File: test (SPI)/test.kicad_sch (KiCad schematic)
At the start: 22 parts, among them J1 Conn_01x02, J2 Conn_01x02, J3 Conn_01x10, U1 DRV8873SPWPRQ1

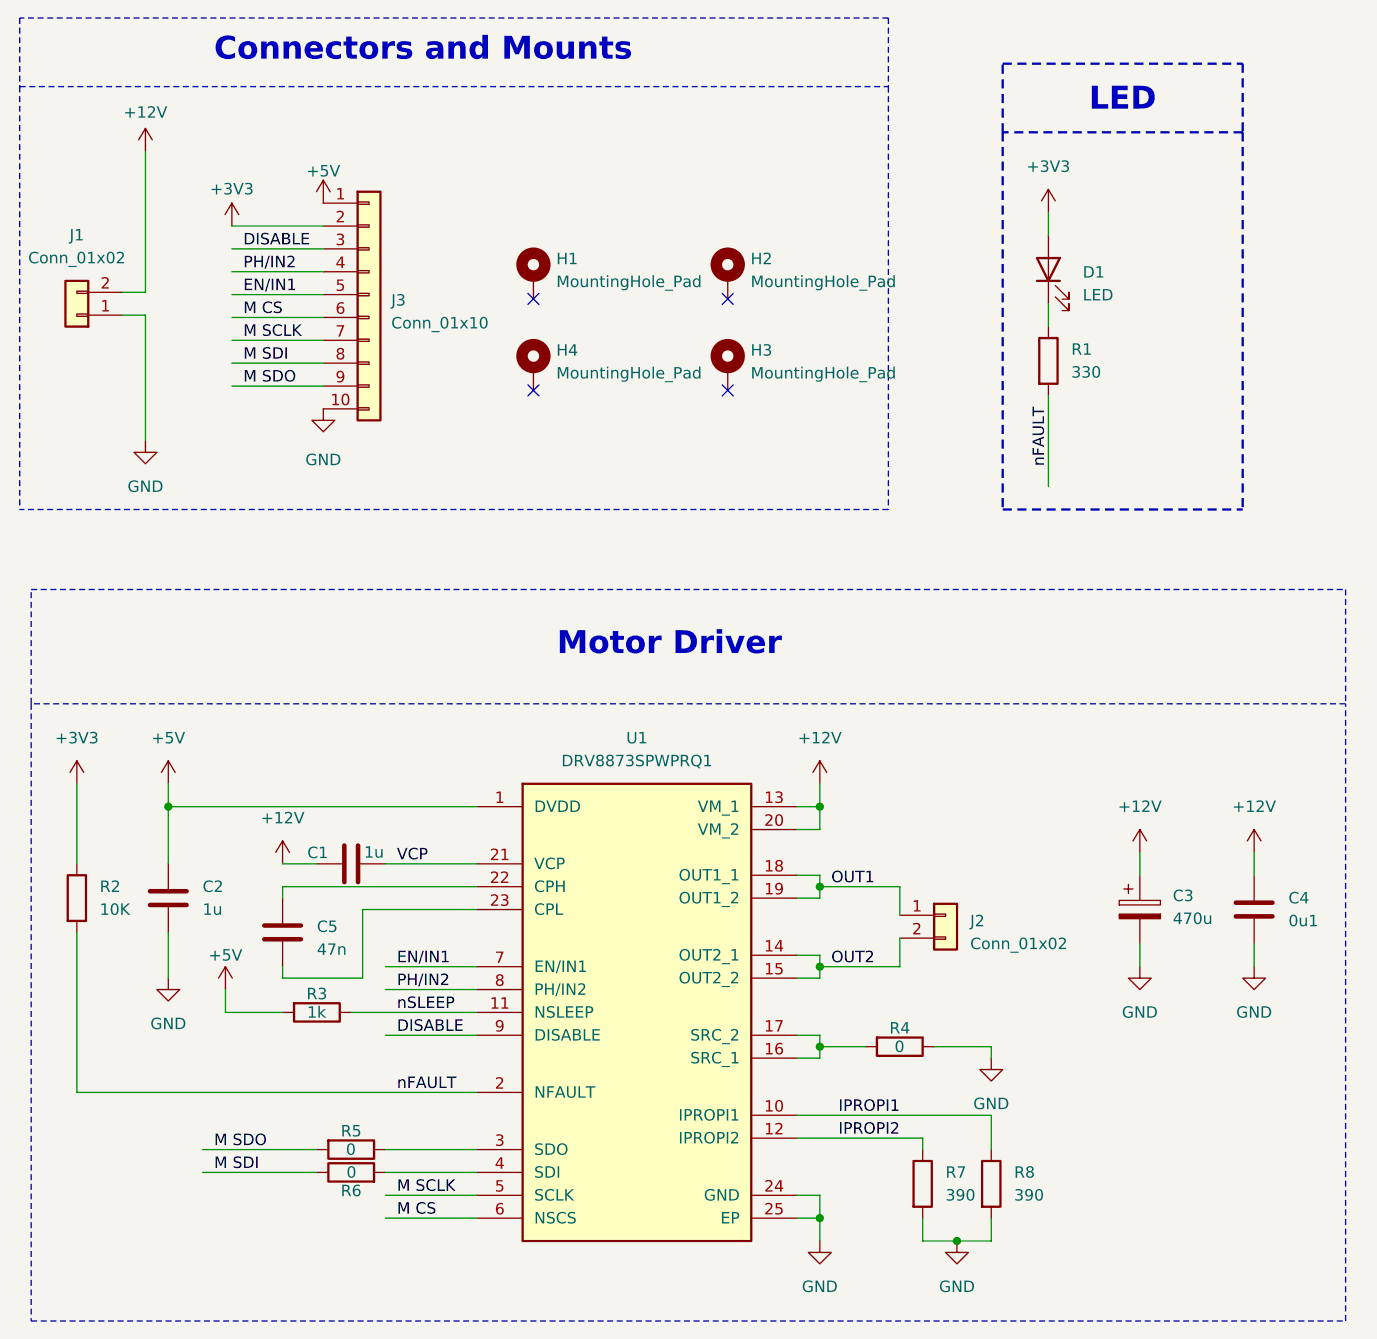
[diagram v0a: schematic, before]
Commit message: Test PCBS
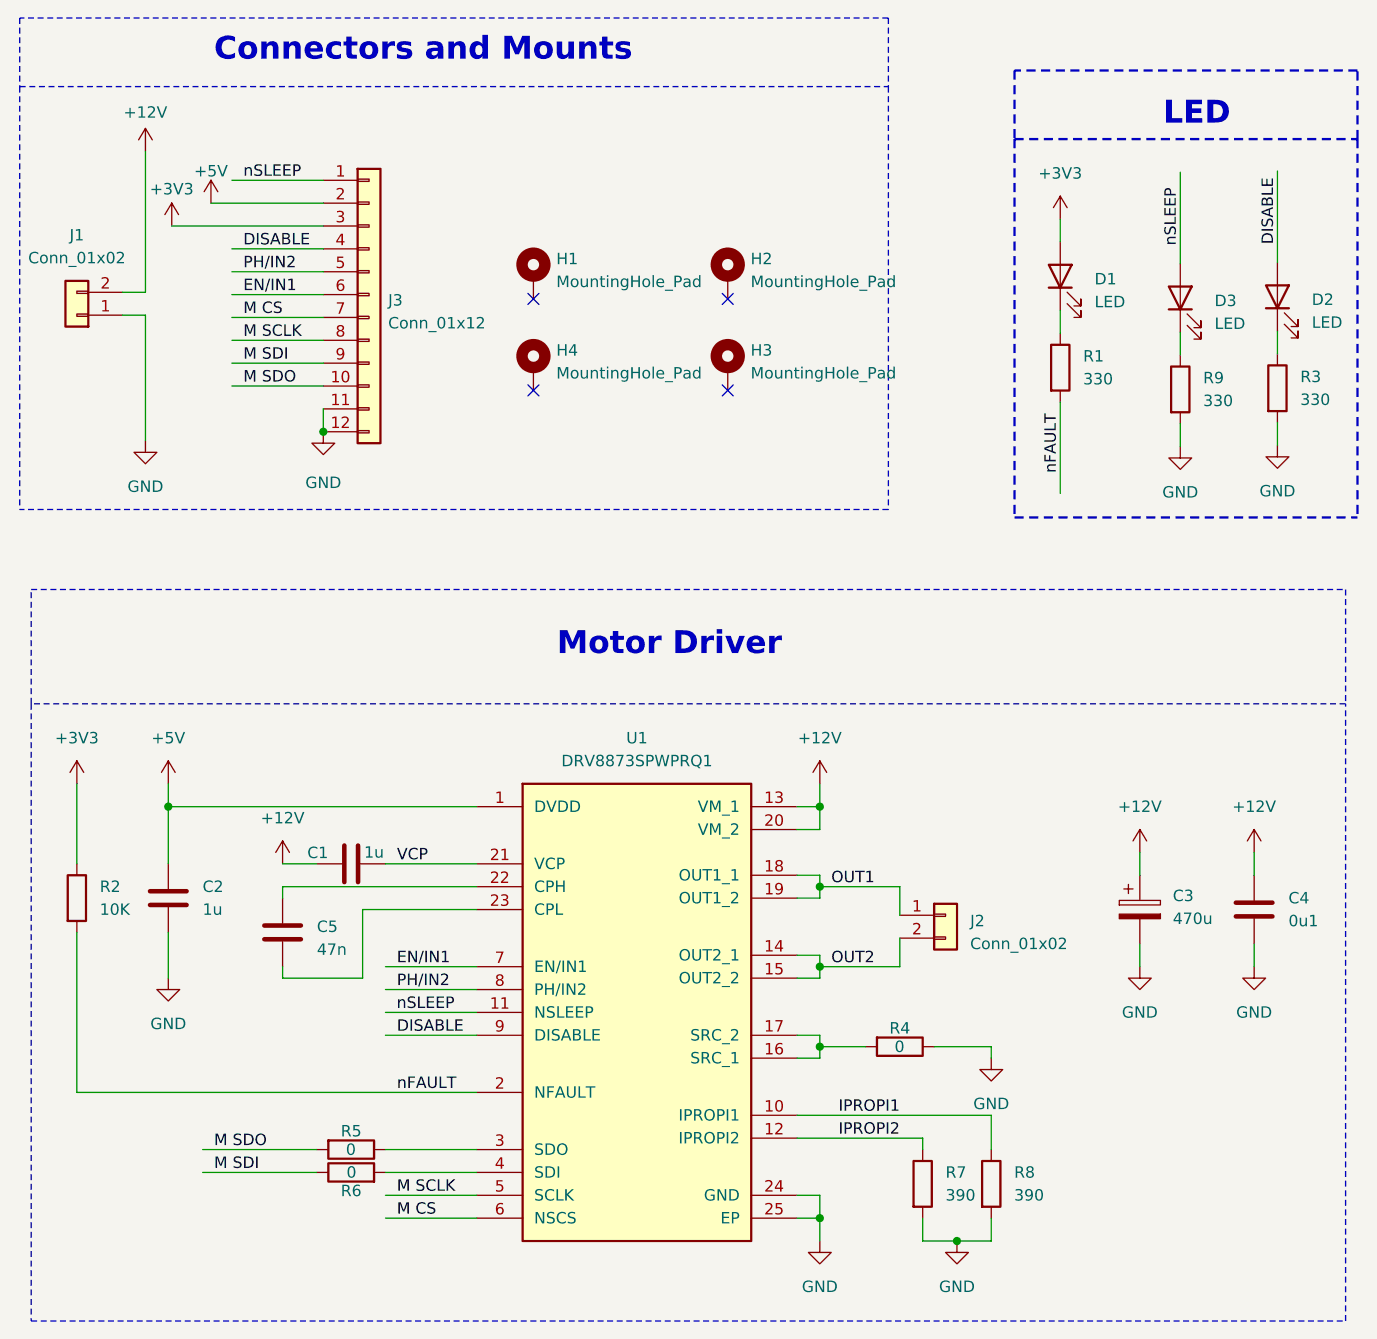
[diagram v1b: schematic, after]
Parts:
- removed J3: Conn_01x10, Connector_PinSocket_2.54mm:PinSocket_1x10_P2.54mm_Vertical, symbol Connector_Generic:Conn_01x10
- added D2, D3: LED, test:led0603, symbol Device:LED
- added J3: Conn_01x12, Connector_PinSocket_2.54mm:PinSocket_1x12_P2.54mm_Vertical, symbol Connector_Generic:Conn_01x12
- added R9: 330, test:res0603, symbol Device:R
- R3: value 1k -> 330
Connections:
- net +3V3: now also J3.3 (Pin_3)
- net +5V: now also J3.2 (Pin_2); no longer R3.2
- net DISABLE: now also D2.2 (A), J3.4 (Pin_4)
- net EN/IN1: now also J3.6 (Pin_6)
- net GND: now also R3.2, J3.11 (Pin_11), J3.12 (Pin_12), R9.2
- net M CS: now also J3.7 (Pin_7)
- net M SCLK: now also J3.8 (Pin_8)
- net M SDI: now also J3.9 (Pin_9)
- net M SDO: now also J3.10 (Pin_10)
- net PH/IN2: now also J3.5 (Pin_5)
- net nSLEEP: now also D3.2 (A), J3.1 (Pin_1); no longer R3.1
- new net: D2.1 (K), R3.1
- new net: D3.1 (K), R9.1
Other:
- note added: "LED"
